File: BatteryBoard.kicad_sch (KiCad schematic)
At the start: 17 parts, among them J1 Keystone-1042, J2 Keystone-1042, J3 Keystone-1042, J4 Keystone-1042, J5 Keystone-1042, J6 Keystone-1042, J7 200528-0120, J8 1985807, J9 1985807, SW1 SW_SPST, SW2 SW_SPST, SW3 SW_SPST, SW4 SW_SPST

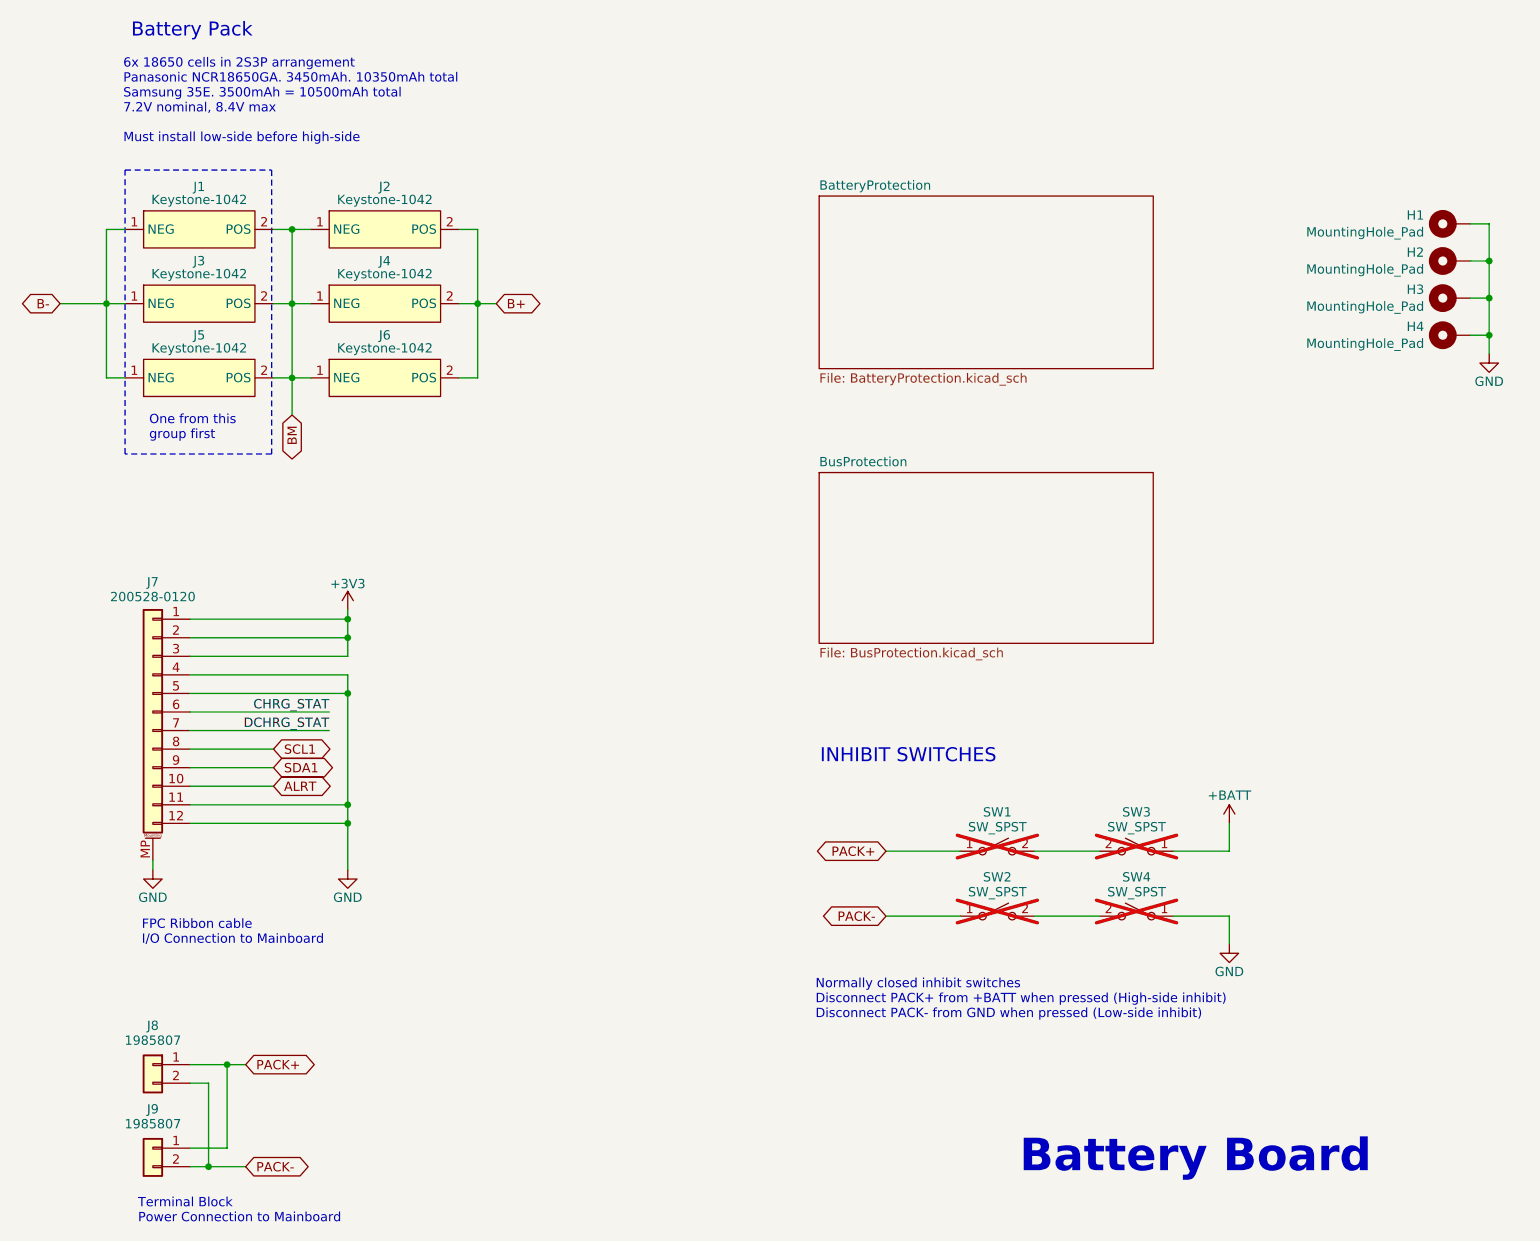
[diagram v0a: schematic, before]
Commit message: Complete layout
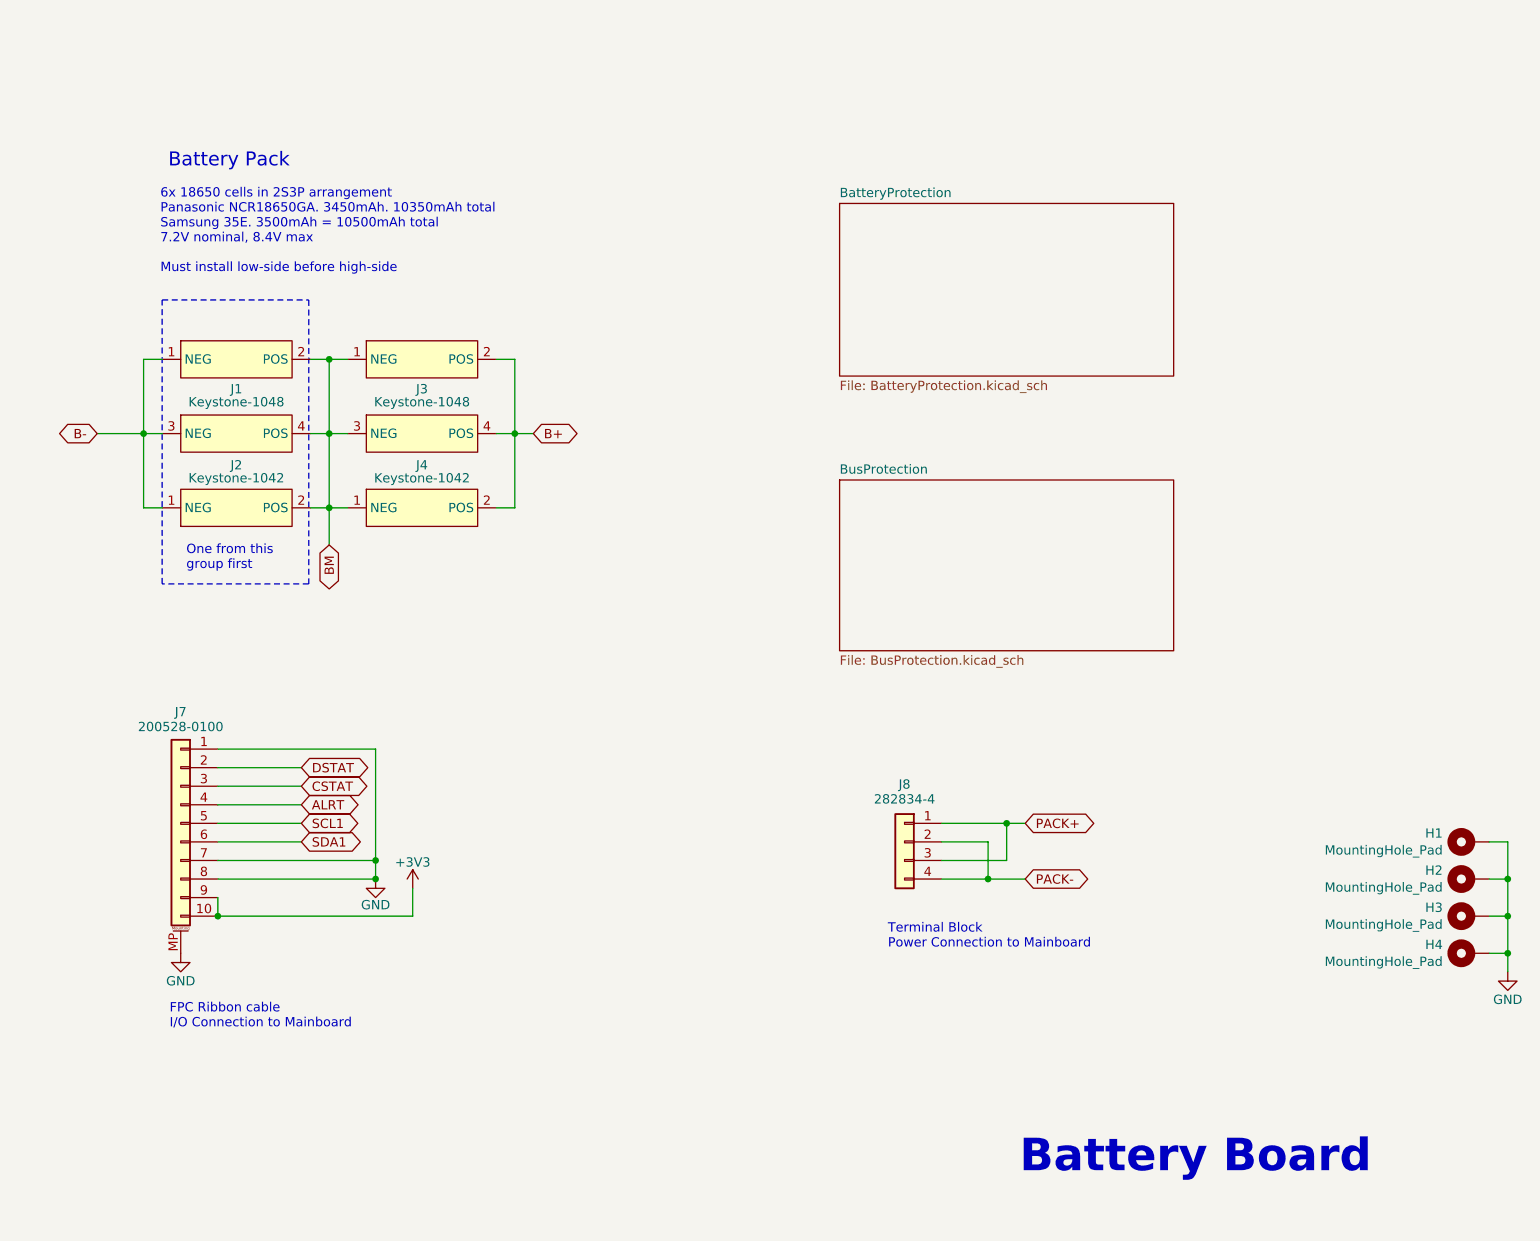
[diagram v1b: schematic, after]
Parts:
- removed J1, J2, J3, J4: Keystone-1042, BatteryBoard:Keystone_1042, symbol BatteryBoard:Keystone-1042
- removed J8, J9: 1985807, symbol Connector_Generic:Conn_01x02
- removed SW1, SW2, SW3, SW4: SW_SPST, symbol Switch:SW_SPST
- added J1, J3: Keystone-1048, BatteryBoard:BAT_1048, symbol BatteryBoard:Keystone-1048
- added J8: 282834-4, BatteryBoard:TE_282834-4, symbol Connector_Generic:Conn_01x04
- J7: value 200528-0120 -> 200528-0100; footprint Connector_FFC-FPC:Molex_200528-0120_1x12-1MP_P1.00mm_Horizontal -> Connector_FFC-FPC:Molex_200528-0100_1x10-1MP_P1.00mm_Horizontal; symbol Connector_Generic_MountingPin:Conn_01x12_MountingPin -> Connector_Generic_MountingPin:Conn_01x10_MountingPin
- renumbered J5 to J2, J6 to J4
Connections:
- net CHRG_STAT is gone; now on net SDA1: J7.6 (Pin_6)
- net DCHRG_STAT is gone; now on net GND: J7.7 (Pin_7)
- net +3V3: now also J7.10 (Pin_10), J7.9 (Pin_9); no longer J7.1 (Pin_1), J7.2 (Pin_2), J7.3 (Pin_3)
- net ALRT: now also J7.4 (Pin_4); no longer J7.10 (Pin_10)
- net B+: now also J3.2 (POS), J3.4 (POS)
- net B-: now also J1.1 (NEG), J1.3 (NEG)
- net BM: now also J1.2 (POS), J1.4 (POS), J3.1 (NEG), J3.3 (NEG)
- net GND: now also J7.1 (Pin_1), J7.8 (Pin_8); no longer J7.11 (Pin_11), J7.12 (Pin_12), J7.4 (Pin_4), J7.5 (Pin_5)
- net PACK+: now also J8.1 (Pin_1), J8.3 (Pin_3)
- net PACK-: now also J8.2 (Pin_2), J8.4 (Pin_4)
- net SCL1: now also J7.5 (Pin_5); no longer J7.8 (Pin_8)
- net SDA1: no longer J7.9 (Pin_9)
- new net CSTAT: J7.3 (Pin_3)
- new net DSTAT: J7.2 (Pin_2)
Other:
- note removed: "INHIBIT SWITCHES"
- note removed: "Normally closed inhibit switches Disconnect PACK+ from +BATT when pressed (High-side inhibit) Disconnect PACK- from GND when pressed (Low-side inhibit)"
- moved on the sheet: H1, H2, H3, H4, J2, J4
